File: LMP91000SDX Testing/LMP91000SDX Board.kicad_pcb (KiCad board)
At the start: 2 copper layers, 16 x 12 mm, 1 part, among them U1 LMP91000SDX/NOPB

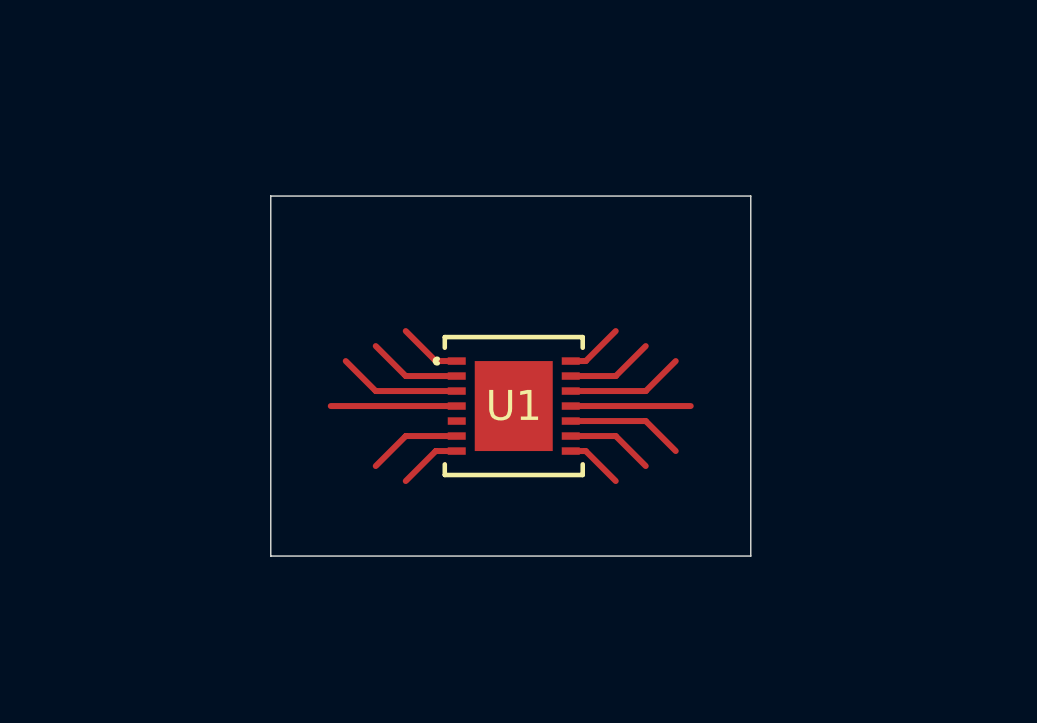
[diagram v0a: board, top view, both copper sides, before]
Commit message: Testing Board Completed
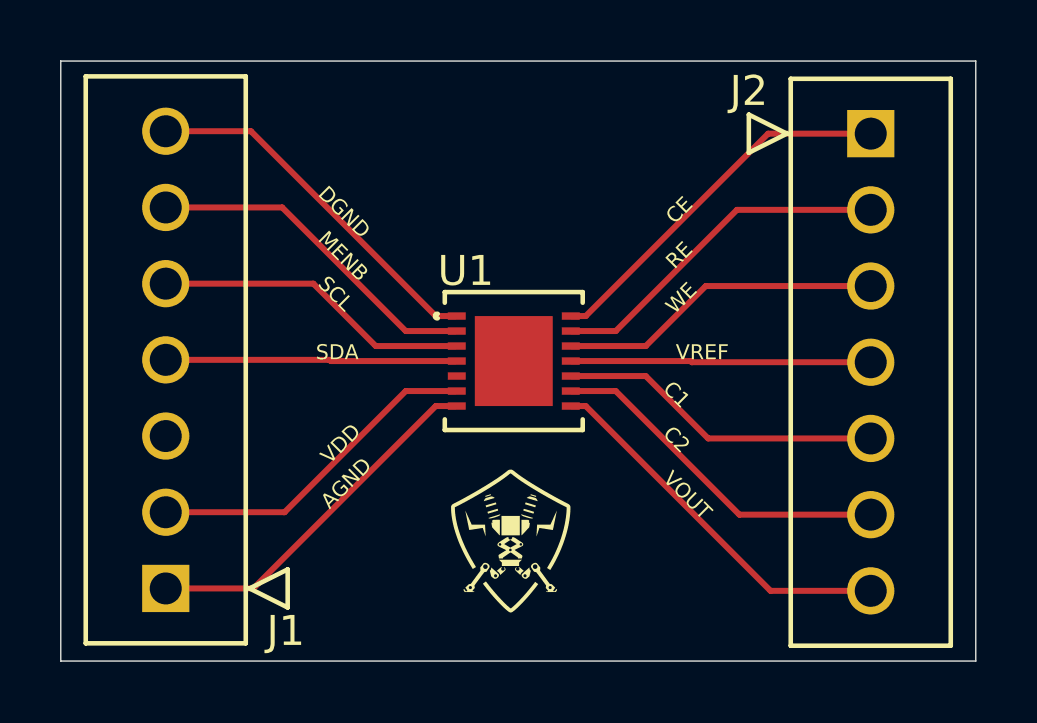
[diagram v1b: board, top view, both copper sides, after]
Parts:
- added G***: LOGO, Pylon:Pylon, F.Cu at (115.0, 113.5)
- added J1: PPTC071LFBN-RC, PPTC071LFBN_RC:CONN_xPxC071LFBN-RC_SUL, F.Cu at (103.5, 115.1)
- added J2: PPTC071LFBN-RC, PPTC071LFBN_RC:CONN_xPxC071LFBN-RC_SUL, F.Cu at (127.0, 99.9)
- moved U1 1.50 mm to (115.1, 107.5)
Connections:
- U1 pad 1: unconnected-(U1-DGND-Pad1) -> Net-(U1-DGND)
- U1 pad 10: unconnected-(U1-C1-Pad10) -> Net-(U1-C1)
- U1 pad 11: unconnected-(U1-VREF-Pad11) -> Net-(U1-VREF)
- U1 pad 12: unconnected-(U1-WE-Pad12) -> Net-(U1-WE)
- U1 pad 13: unconnected-(U1-RE-Pad13) -> Net-(U1-RE)
- U1 pad 14: unconnected-(U1-CE-Pad14) -> Net-(U1-CE)
- U1 pad 2: unconnected-(U1-MENB-Pad2) -> Net-(U1-MENB)
- U1 pad 3: unconnected-(U1-SCL-Pad3) -> Net-(U1-SCL)
- U1 pad 4: unconnected-(U1-SDA-Pad4) -> Net-(U1-SDA)
- U1 pad 6: unconnected-(U1-VDD-Pad6) -> Net-(U1-VDD)
- U1 pad 7: unconnected-(U1-AGND-Pad7) -> Net-(U1-AGND)
- U1 pad 8: unconnected-(U1-VOUT-Pad8) -> Net-(U1-VOUT)
- U1 pad 9: unconnected-(U1-C2-Pad9) -> Net-(U1-C2)
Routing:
- net Net-(U1-VOUT): track 0.00 -> 12.6 mm
- net Net-(U1-CE): track 0.00 -> 12.5 mm
- net Net-(U1-DGND): track 0.00 -> 12.3 mm
- net Net-(U1-AGND): track 0.00 -> 12.2 mm
- net Net-(U1-C2): track 0.00 -> 11.7 mm
- net Net-(U1-RE): track 0.00 -> 11.7 mm
- net Net-(U1-MENB): track 0.00 -> 11.4 mm
- net Net-(U1-VDD): track 0.00 -> 11.4 mm
- net Net-(U1-C1): track 0.00 -> 10.9 mm
- net Net-(U1-WE): track 0.00 -> 10.8 mm
- net Net-(U1-SCL): track 0.00 -> 10.6 mm
- net Net-(U1-VREF): track 0.00 -> 10.0 mm
- net Net-(U1-SDA): track 0.00 -> 9.72 mm
- net unconnected-(U1-SDA-Pad4): track 4.20 -> 0.00 mm
- net unconnected-(U1-SCL-Pad3): track 4.11 -> 0.00 mm
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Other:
- board size 16 x 12 mm -> 30.5 x 20 mm
- board text added: "AGND"
- board text added: "C1"
- board text added: "C2"
- board text added: "CE"
- board text added: "DGND"
- board text added: "MENB"
- board text added: "RE"
- board text added: "SCL"
- board text added: "SDA"
- board text added: "VDD"
- board text added: "VOUT"
- board text added: "VREF"
- board text added: "WE"
